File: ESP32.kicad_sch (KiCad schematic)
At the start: 13 parts, among them J7 USB_C_Receptacle_USB2.0_16P, Q1 SS8050, Q2 SS8050, U2 ESP32-WROOM-32U, U4 CH340C

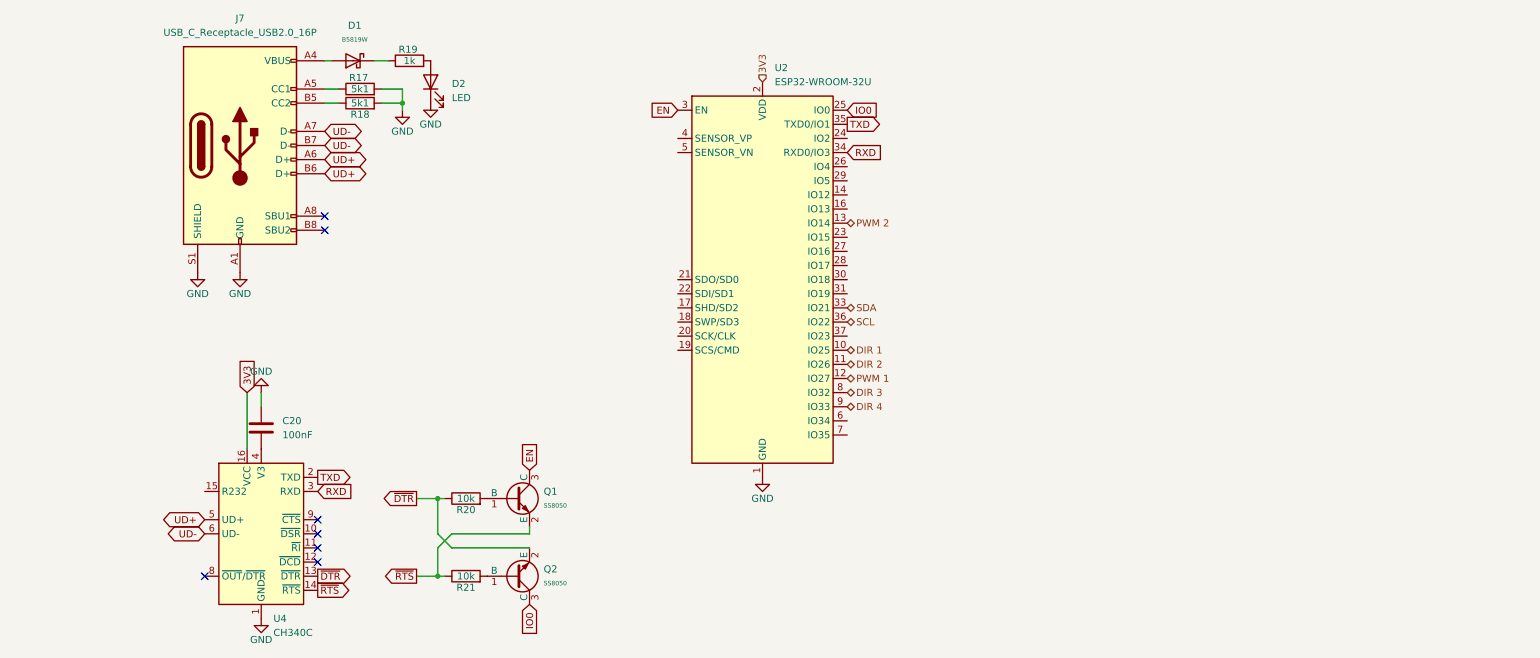
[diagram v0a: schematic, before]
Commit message: Schematic V1
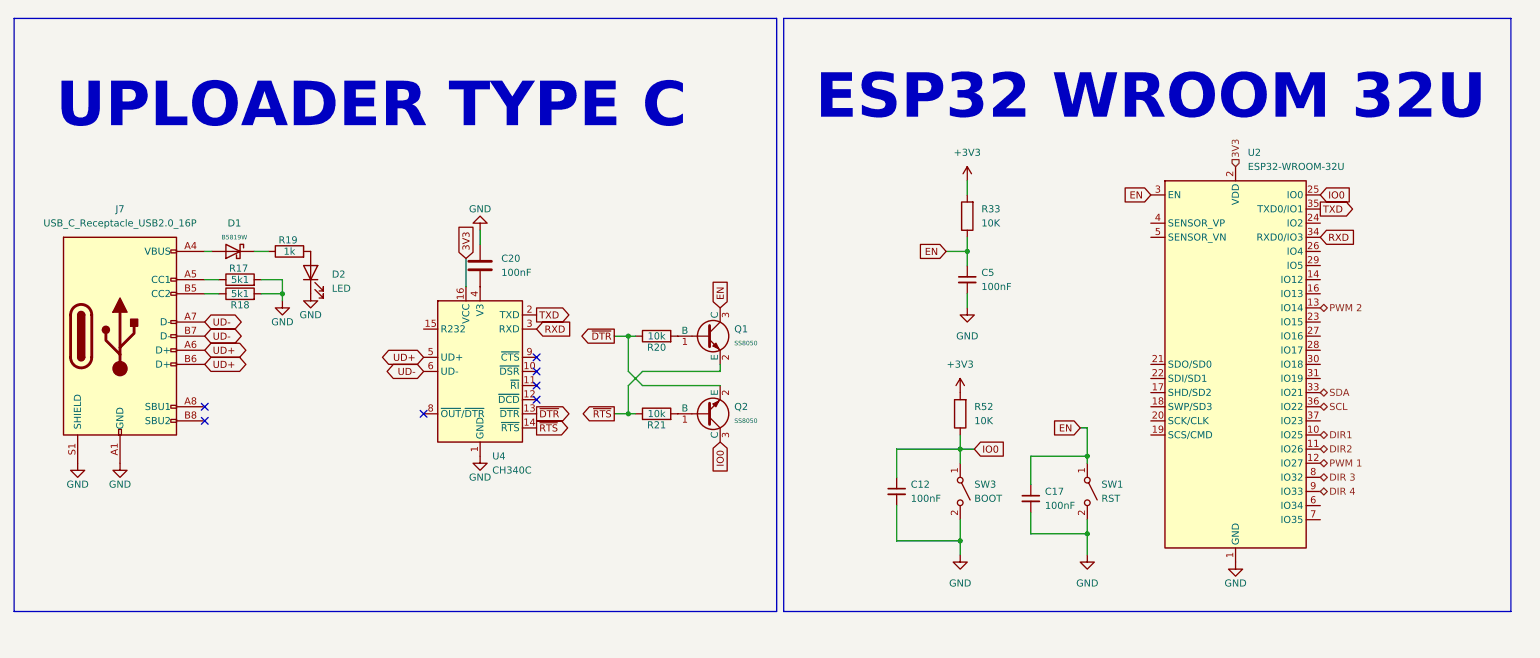
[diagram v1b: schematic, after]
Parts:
- added C12, C17, C5: 100nF, Capacitor_SMD:C_0805_2012Metric_Pad1.18x1.45mm_HandSolder, symbol Device:C_Small
- added R33, R52: 10K, Resistor_SMD:R_0805_2012Metric_Pad1.20x1.40mm_HandSolder, symbol Device:R
- added SW1: RST, Button_Switch_SMD:SW_SPST_CK_RS282G05A3, symbol Switch:SW_SPST
- added SW3: BOOT, Button_Switch_SMD:SW_SPST_CK_RS282G05A3, symbol Switch:SW_SPST
- D1: footprint PCM_JLCPCB:D_SOD-123 -> Diode_SMD:Nexperia_CFP3_SOD-123W
- D2: footprint (none) -> LED_SMD:LED_1206_3216Metric_Pad1.42x1.75mm_HandSolder
- Q1, Q2: footprint PCM_JLCPCB:Q_SOT-23 -> Package_TO_SOT_SMD:SOT-23_Handsoldering
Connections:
- net EN: now also C17.1, C5.1, R33.1, SW1.1 (A)
- net GND: now also C12.2, C17.2, C5.2, SW1.2 (B), SW3.2 (B)
- net IO0: now also C12.1, R52.1, SW3.1 (A)
- net DIR 1 renamed DIR1
- net DIR 2 renamed DIR2
- new net +3V3: R33.2, R52.2
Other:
- note added: "ESP32 WROOM 32U"
- note added: "UPLOADER TYPE C"
- title: Board Robot SUMO -> Board Robot SOCCER & SUMO
- moved on the sheet: C20, D1, D2, J7, Q1, Q2, R17, R18, R19, R20, R21, U2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
